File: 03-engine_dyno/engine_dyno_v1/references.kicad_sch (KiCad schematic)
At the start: 4 parts, among them U5 AD5689RBRUZ

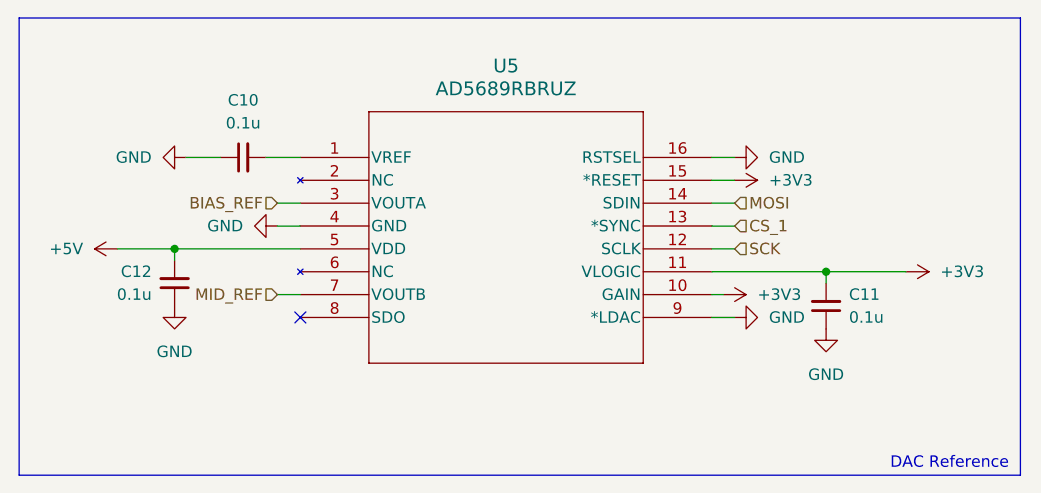
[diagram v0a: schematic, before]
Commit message: minor changes
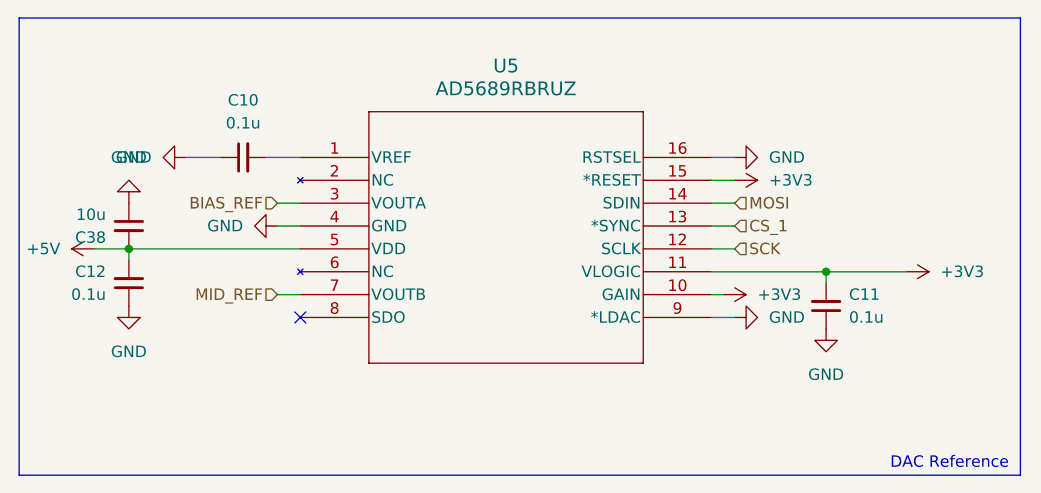
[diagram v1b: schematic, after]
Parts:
- added C38: 10u, Capacitor_SMD:C_0402_1005Metric, symbol Device:C_Small
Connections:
- net +5V: now also C38.2
- net GND: now also C38.1
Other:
- moved on the sheet: C12
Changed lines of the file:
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@@
 	)
 	(junction
-		(at 113.03 102.87)
+		(at 107.95 102.87)
 		(diameter 0)
 		(color 0 0 0 0)
@@
 	(wire
 		(pts
-			(xy 113.03 102.87) (xy 113.03 104.14)
+			(xy 107.95 102.87) (xy 107.95 104.14)
 		)
 		(stroke
@@
 	(wire
 		(pts
+			(xy 107.95 102.87) (xy 127 102.87)
+		)
+		(stroke
+			(width 0)
+			(type default)
+		)
+	)
+	(wire
+		(pts
 			(xy 173.99 107.95) (xy 172.72 107.95)
 		)
@@
 	(wire
 		(pts
-			(xy 106.68 102.87) (xy 113.03 102.87)
+			(xy 104.14 102.87) (xy 107.95 102.87)
 		)
 		(stroke
@@
 		(pts
 			(xy 172.72 102.87) (xy 175.26 102.87)
-		)
-		(stroke
-			(width 0)
-			(type default)
-		)
-	)
-	(wire
-		(pts
-			(xy 113.03 102.87) (xy 127 102.87)
 		)
 		(stroke
@@
 	)
 	(symbol
+		(lib_id "Device:C_Small")
+		(at 107.95 100.33 0)
+		(unit 1)
+		(exclude_from_sim no)
+		(in_bom yes)
+		(on_board yes)
+		(dnp no)
+		(property "Reference" "C38"
+			(at 105.41 101.6065 0)
+			(effects
+				(font
+					(size 1.27 1.27)
+				)
+				(justify right)
+			)
+		)
+		(property "Value" "10u"
+			(at 105.41 99.0665 0)
+			(effects
+				(font
+					(size 1.27 1.27)
+				)
+				(justify right)
+			)
+		)
+		(property "Footprint" "Capacitor_SMD:C_0402_1005Metric"
+			(at 107.95 100.33 0)
+			(effects
+				(font
+					(size 1.27 1.27)
+				)
+				(hide yes)
+			)
+		)
+		(property "Datasheet" "~"
+			(at 107.95 100.33 0)
+			(effects
+				(font
+					(size 1.27 1.27)
+				)
+				(hide yes)
+			)
+		)
+		(property "Description" "Unpolarized capacitor, small symbol"
+			(at 107.95 100.33 0)
+			(effects
+				(font
+					(size 1.27 1.27)
+				)
+				(hide yes)
+			)
+		)
+		(pin "1"
+		)
+		(pin "2"
+		)
+		(instances
+			(project "engine_dyno_v1"
+				(path "/d283b024-74fa-4d4c-9089-b2007a8f756c/0c6943d1-72c8-4350-bd84-a52e2c8b9947"
+					(reference "C38")
+					(unit 1)
+				)
+			)
+		)
+	)
+	(symbol
 		(lib_id "AD5689R:AD5689RBRUZ")
 		(at 127 92.71 0)
@@
 	(symbol
 		(lib_id "power:GND")
-		(at 113.03 109.22 0)
+		(at 107.95 109.22 0)
 		(unit 1)
 		(exclude_from_sim no)
@@
 		(fields_autoplaced yes)
 		(property "Reference" "#PWR040"
-			(at 113.03 115.57 0)
+			(at 107.95 115.57 0)
 			(effects
 				(font
@@
 		)
 		(property "Value" "GND"
-			(at 113.03 114.3 0)
+			(at 107.95 114.3 0)
 			(effects
 				(font
@@
 		)
 		(property "Footprint" ""
-			(at 113.03 109.22 0)
+			(at 107.95 109.22 0)
 			(effects
 				(font
@@
 		)
 		(property "Datasheet" ""
-			(at 113.03 109.22 0)
+			(at 107.95 109.22 0)
 			(effects
 				(font
@@
 		)
 		(property "Description" "Power symbol creates a global label with name \"GND\" , ground"
-			(at 113.03 109.22 0)
+			(at 107.95 109.22 0)
 			(effects
 				(font
@@
 	(symbol
 		(lib_id "power:+5V")
-		(at 106.68 102.87 90)
+		(at 104.14 102.87 90)
 		(unit 1)
 		(exclude_from_sim no)
@@
 		(fields_autoplaced yes)
 		(property "Reference" "#PWR032"
-			(at 110.49 102.87 0)
+			(at 107.95 102.87 0)
 			(effects
 				(font
@@
 		)
 		(property "Value" "+5V"
-			(at 102.87 102.8699 90)
+			(at 100.33 102.8699 90)
 			(effects
 				(font
@@
 		)
 		(property "Footprint" ""
-			(at 106.68 102.87 0)
+			(at 104.14 102.87 0)
 			(effects
 				(font
@@
 		)
 		(property "Datasheet" ""
-			(at 106.68 102.87 0)
+			(at 104.14 102.87 0)
 			(effects
 				(font
@@
 		)
 		(property "Description" "Power symbol creates a global label with name \"+5V\""
-			(at 106.68 102.87 0)
+			(at 104.14 102.87 0)
 			(effects
 				(font
@@
 				(path "/d283b024-74fa-4d4c-9089-b2007a8f756c/0c6943d1-72c8-4350-bd84-a52e2c8b9947"
 					(reference "#PWR032")
+					(unit 1)
+				)
+			)
+		)
+	)
+	(symbol
+		(lib_id "power:GND")
+		(at 107.95 97.79 0)
+		(mirror x)
+		(unit 1)
+		(exclude_from_sim no)
+		(in_bom yes)
+		(on_board yes)
+		(dnp no)
+		(fields_autoplaced yes)
+		(property "Reference" "#PWR055"
+			(at 107.95 91.44 0)
+			(effects
+				(font
+					(size 1.27 1.27)
+				)
+				(hide yes)
+			)
+		)
+		(property "Value" "GND"
+			(at 107.95 92.71 0)
+			(effects
+				(font
+					(size 1.27 1.27)
+				)
+			)
+		)
+		(property "Footprint" ""
+			(at 107.95 97.79 0)
+			(effects
+				(font
+					(size 1.27 1.27)
+				)
+				(hide yes)
+			)
+		)
+		(property "Datasheet" ""
+			(at 107.95 97.79 0)
+			(effects
+				(font
+					(size 1.27 1.27)
+				)
+				(hide yes)
+			)
+		)
+		(property "Description" "Power symbol creates a global label with name \"GND\" , ground"
+			(at 107.95 97.79 0)
+			(effects
+				(font
+					(size 1.27 1.27)
+				)
+				(hide yes)
+			)
+		)
+		(pin "1"
+		)
+		(instances
+			(project "engine_dyno_v1"
+				(path "/d283b024-74fa-4d4c-9089-b2007a8f756c/0c6943d1-72c8-4350-bd84-a52e2c8b9947"
+					(reference "#PWR055")
 					(unit 1)
 				)
@@
 	(symbol
 		(lib_id "Device:C_Small")
-		(at 113.03 106.68 0)
+		(at 107.95 106.68 0)
 		(mirror x)
 		(unit 1)
@@
 		(dnp no)
 		(property "Reference" "C12"
-			(at 110.49 105.4035 0)
+			(at 105.41 105.4035 0)
 			(effects
 				(font
@@
 		)
 		(property "Value" "0.1u"
-			(at 110.49 107.9435 0)
+			(at 105.41 107.9435 0)
 			(effects
 				(font
@@
 		)
 		(property "Footprint" "Capacitor_SMD:C_0402_1005Metric"
-			(at 113.03 106.68 0)
+			(at 107.95 106.68 0)
 			(effects
 				(font
@@
 		)
 		(property "Datasheet" "~"
-			(at 113.03 106.68 0)
+			(at 107.95 106.68 0)
 			(effects
 				(font
@@
 		)
 		(property "Description" "Unpolarized capacitor, small symbol"
-			(at 113.03 106.68 0)
-			(effects
-				(font
+			(at 107.95 106.68 0)
+			(effects
+				(font

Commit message: some more changes
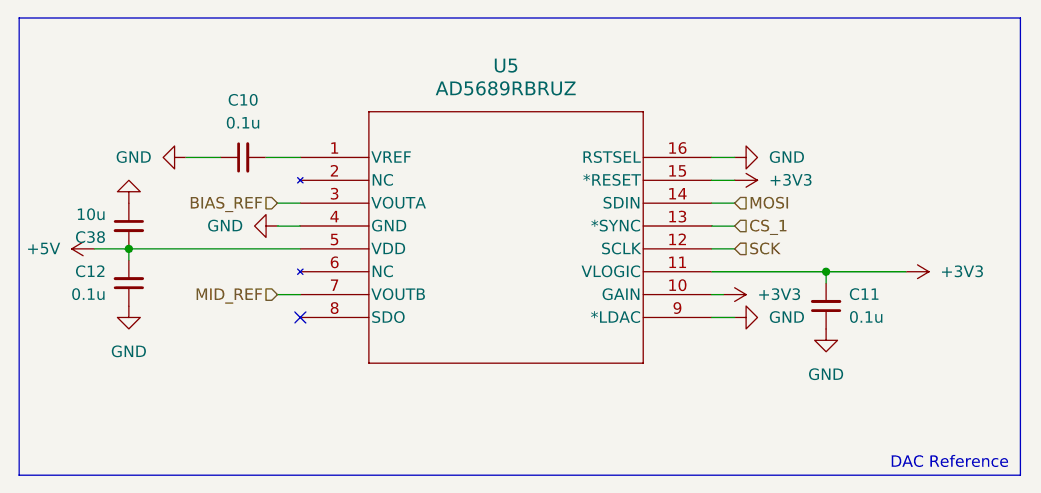
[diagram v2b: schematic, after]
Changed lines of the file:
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@@
 					(size 1.27 1.27)
 				)
+				(hide yes)
 			)
 		)
